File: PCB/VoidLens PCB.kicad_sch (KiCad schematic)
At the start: 75 parts, among them IC1 BMI270, J1 solder pad, J2 JST-XH-2 Pin, J4 JST_XH for led Strip, J5 Programming_Pins, SW1 K3-1391A, SW2 SW_Push_DPDT, SW5 K2-1157SP-I4SW-04, U1 BQ24074RGT, U2 ATmega32U4-M, U3 NRF24L01, U5 TPS61022, U6 TPS27081ADDCR, Y1 16Mhz, Y2 16mhz

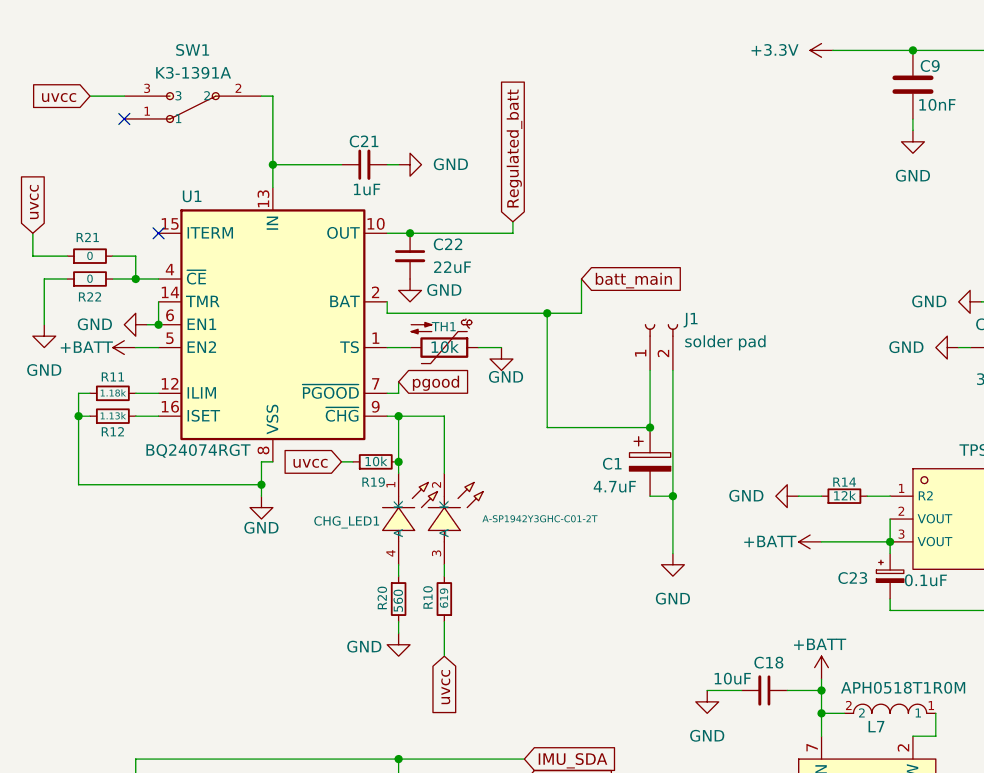
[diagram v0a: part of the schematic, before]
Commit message: Arrangeed components to their positions in pcb
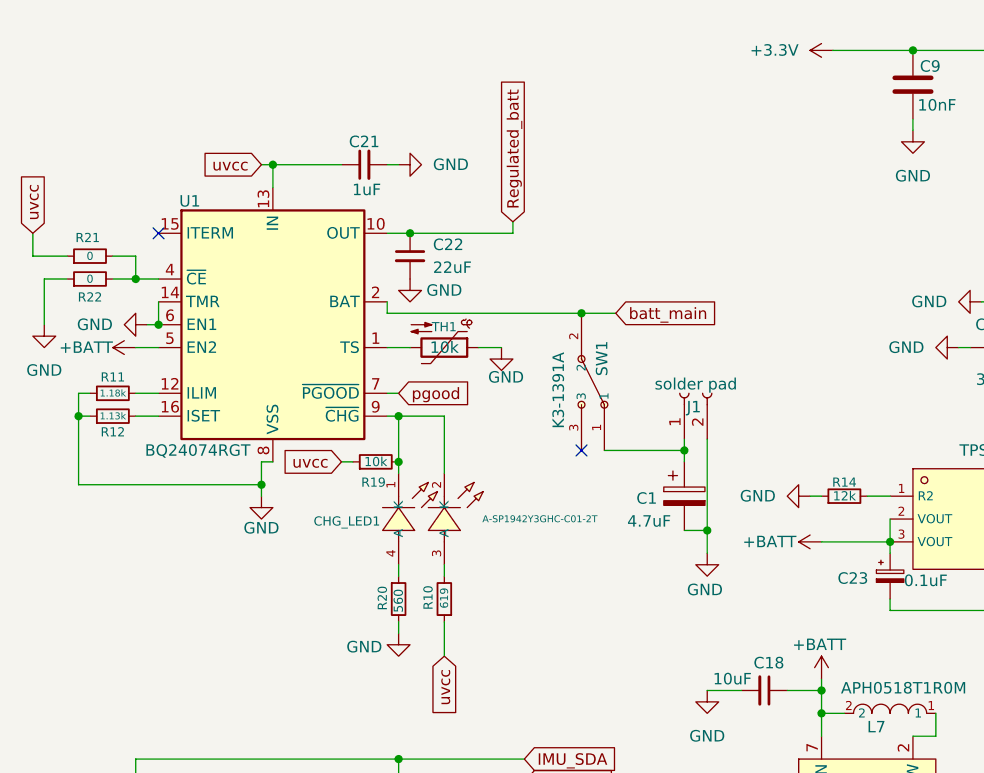
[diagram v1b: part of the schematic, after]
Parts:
- C22: footprint Capacitor_SMD:C_0603_1608Metric_Pad1.08x0.95mm_HandSolder -> Capacitor_SMD:CP_Elec_4x5.4
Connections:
- net batt_main: now also SW1.2; no longer C1.1, J1.1 (Pin_1)
- net uvcc: now also C21.1, U1.13 (IN); no longer SW1.3
- net at SW1.1: now also C1.1, J1.1 (Pin_1)
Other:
- moved on the sheet: C1, J1
